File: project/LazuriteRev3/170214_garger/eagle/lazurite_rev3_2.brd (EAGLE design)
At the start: 76.2 x 53.3 mm, 62 parts, among them IC1 FT232RQ

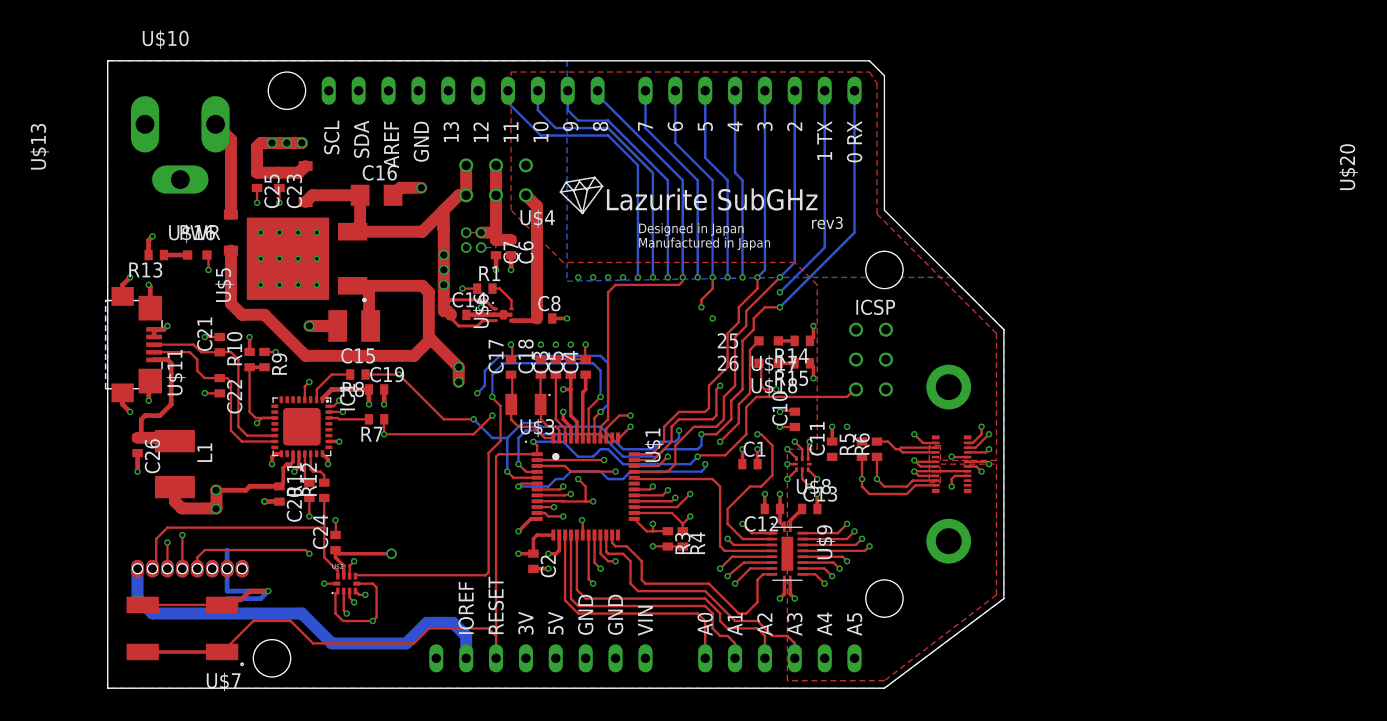
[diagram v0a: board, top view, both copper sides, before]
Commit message: update libraries and projects
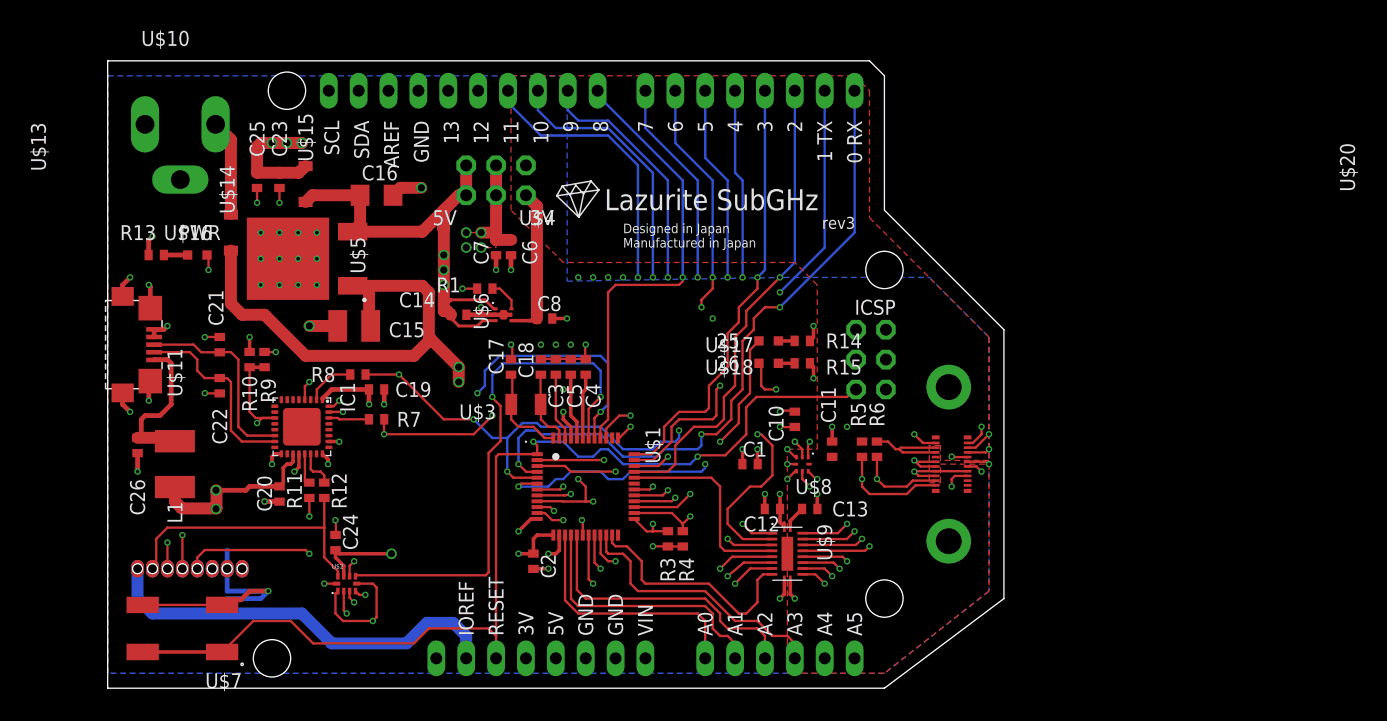
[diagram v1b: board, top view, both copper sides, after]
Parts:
- U$8: device lazurite:FXMA2102 -> lazurite:MICROPACK
- moved U$19 0.45 mm to (37.5, 41.9)
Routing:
- net P45: track 71.1 -> 71.6 mm
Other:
- board text added: "3V"
- board text added: "5V"
